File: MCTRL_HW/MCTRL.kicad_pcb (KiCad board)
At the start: 2 copper layers, 70 x 50 mm, 21 parts, among them J1 393570004, J2 393570004, J3 393570004, U1 IR2110, U2 IR2110, U3 IPD70R360P7SAUMA1, U4 IPD70R360P7SAUMA1, U5 IPD70R360P7SAUMA1, U6 IPD70R360P7SAUMA1

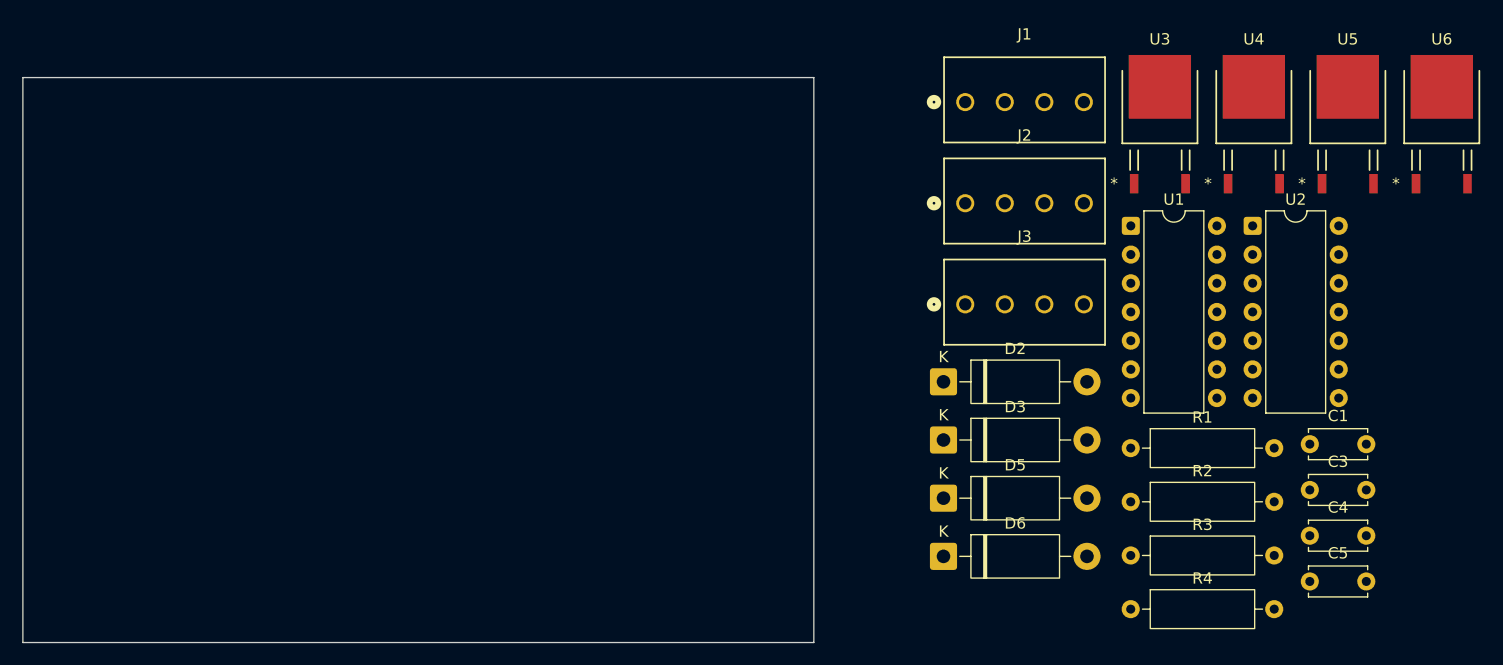
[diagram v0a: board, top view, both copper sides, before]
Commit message: Unfinished PCB
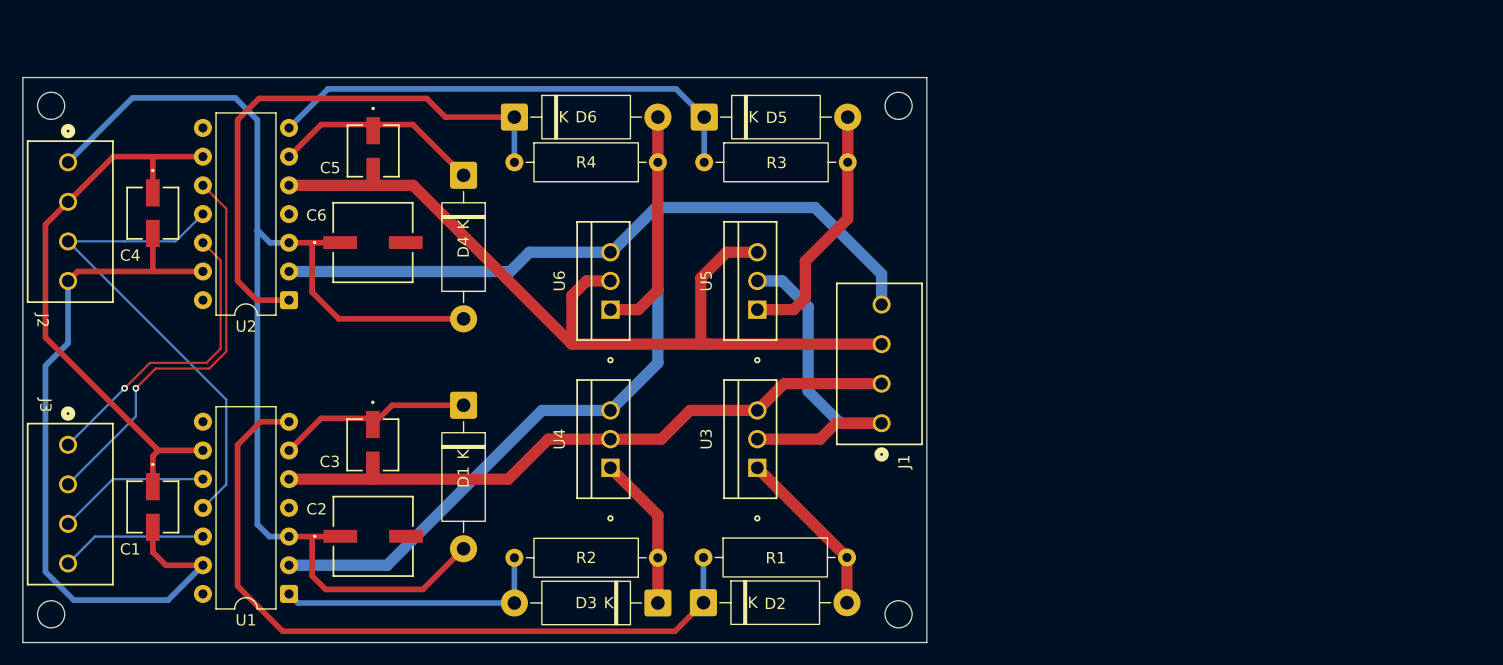
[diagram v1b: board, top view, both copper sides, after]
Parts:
- added C2: 22u, MCTRL:EEEFK1H220P, F.Cu at (151.0, 120.6)
- added C6: 22u, MCTRL:EEEFK1H220P, F.Cu at (151.0, 94.6)
- added D1: UF4007, Diode_THT:D_DO-15_P12.70mm_Horizontal, F.Cu at (159.0, 109.0)
- added D4: UF4007, Diode_THT:D_DO-15_P12.70mm_Horizontal, F.Cu at (159.0, 88.7)
- C1, C4: footprint Capacitor_THT:C_Disc_D5.0mm_W2.5mm_P5.00mm -> MCTRL:UUP1H0R1MCL1GS
- C3, C5: footprint Capacitor_THT:C_Disc_D5.0mm_W2.5mm_P5.00mm -> MCTRL:UWP1HR22MCL1GB
- U3, U4, U5, U6: value IPD70R360P7SAUMA1 -> IPAN60R125PFD7SXKSA1; footprint MCTRL:IPD70R360P7SAUMA1 -> MCTRL:IPAN60R125PFD7SXKSA1
- moved C4 106.3 mm to (131.5, 92.0), turned to -90 degrees
- moved C1 102.5 mm to (131.5, 118.0), turned to -90 degrees
- moved C5 91.2 mm to (151.0, 86.5), turned to -90 degrees
- moved U2 85.5 mm to (143.6, 99.7), turned to 180 degrees
- moved C3 83.0 mm to (151.0, 112.5), turned to -90 degrees
- moved U1 81.3 mm to (143.6, 125.7), turned to 180 degrees
- moved J3 80.4 mm to (124.0, 112.5), turned to -90 degrees
- moved J2 79.5 mm to (124.0, 87.5), turned to -90 degrees
- moved U6 75.7 mm to (172.0, 100.5), turned to 90 degrees
- moved R4 67.4 mm to (163.5, 87.5)
- moved U4 65.3 mm to (172.0, 114.5), turned to 90 degrees
- moved U5 55.2 mm to (185.0, 100.5), turned to 90 degrees
- moved D6 54.3 mm to (163.5, 83.5)
- moved R3 51.3 mm to (180.3, 87.5)
- moved U3 47.8 mm to (185.0, 114.5), turned to 90 degrees
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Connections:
- J2 pad 1: +3.3V -> +10V
- J2 pad 2: +10V -> +3.3V
- J3 pad 1: Net-(U1-HIN) -> Net-(U2-LIN)
- J3 pad 2: Net-(U1-LIN) -> Net-(U2-HIN)
- J3 pad 3: Net-(U2-HIN) -> Net-(U1-HIN)
- J3 pad 4: Net-(U2-LIN) -> Net-(U1-LIN)
- U1 pad 1: Net-(D3-K) -> Net-(D3-A)
- U4 pad 1: Net-(D3-A) -> Net-(D3-K)
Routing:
- net COM: track 0.00 -> 113.9 mm
- net +10V: track 0.00 -> 108.9 mm
- net Net-(U2-VS): track 0.00 -> 79.5 mm
- net Net-(D2-K): track 0.00 -> 65.9 mm
- net VSS: track 0.00 -> 65.6 mm
- net Net-(U1-VS): track 0.00 -> 57.2 mm
- net +3.3V: track 0.00 -> 51.1 mm
- net Net-(D6-K): track 0.00 -> 49.5 mm
- net Net-(D5-K): track 0.00 -> 43.2 mm
- net Net-(U1-SD): track 0.00 -> 43.2 mm
- net Net-(U2-HIN): track 0.00 -> 35.9 mm, vias 0 -> 1
- net +VDD: track 0.00 -> 32.2 mm
- net Net-(U2-LIN): track 0.00 -> 27.0 mm, vias 0 -> 1
- net Net-(D3-A): track 0.00 -> 24.4 mm
- net Net-(D5-A): track 0.00 -> 22.2 mm
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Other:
- board size 70 x 50 mm -> 80 x 50 mm
